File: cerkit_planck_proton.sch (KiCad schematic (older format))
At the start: 1 part

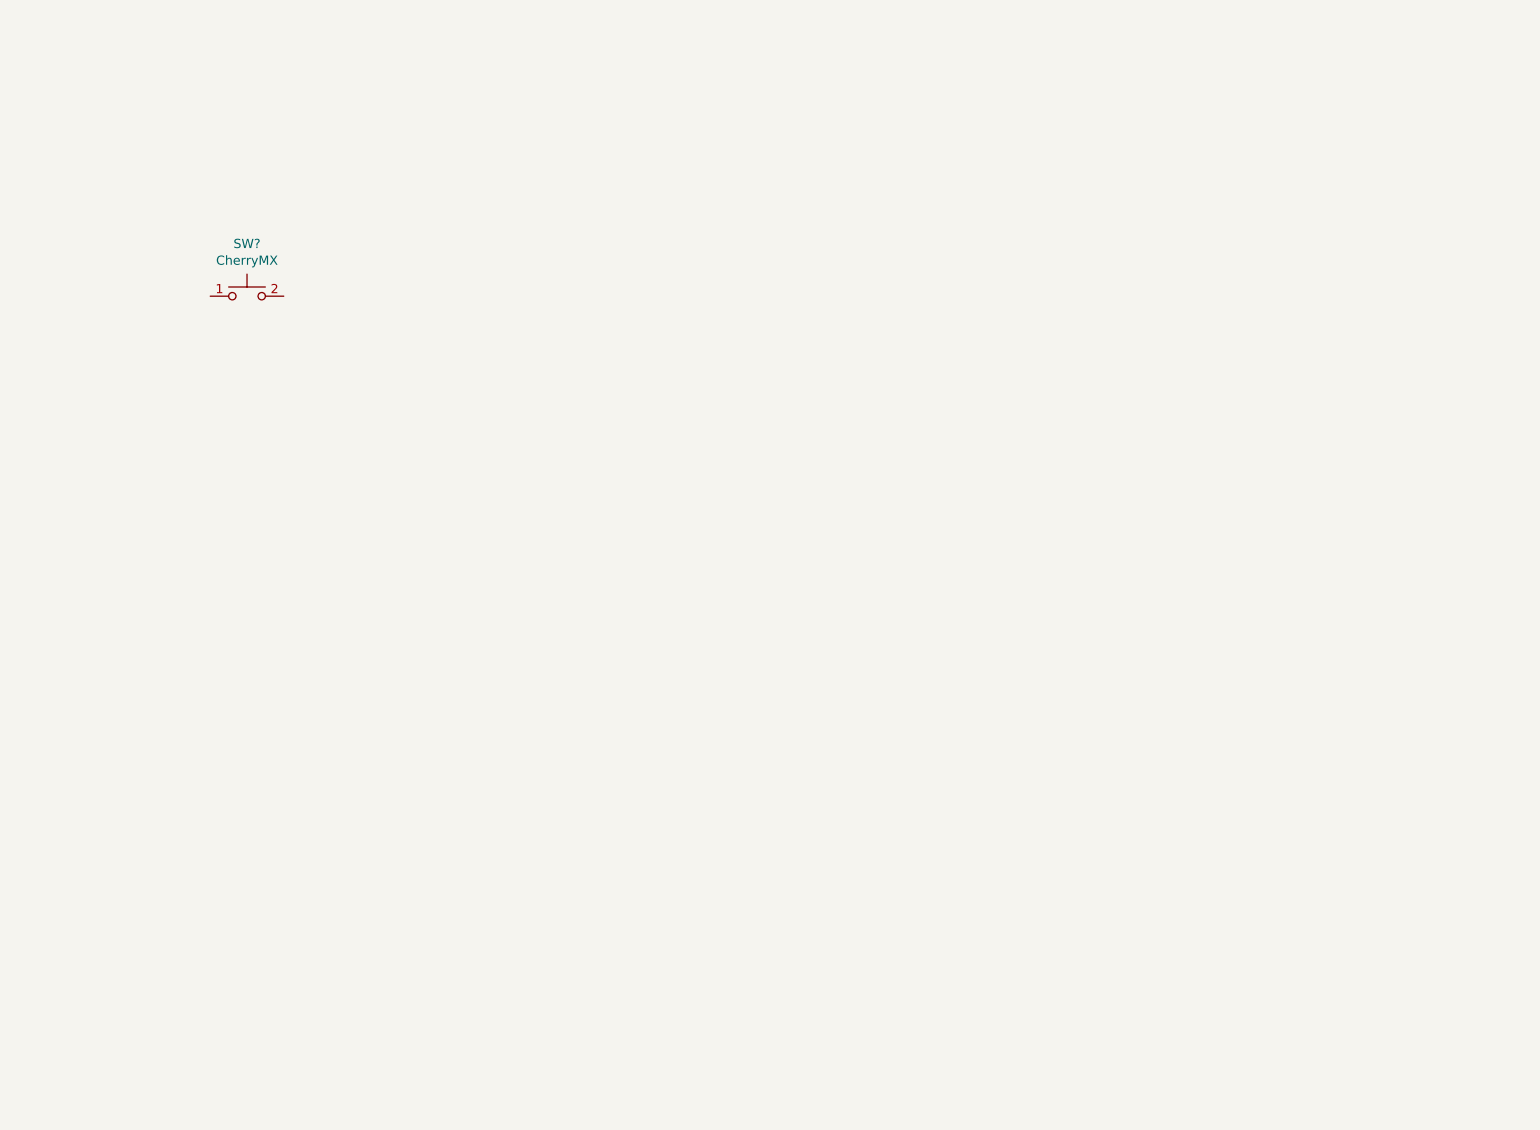
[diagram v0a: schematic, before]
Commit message: added schematic
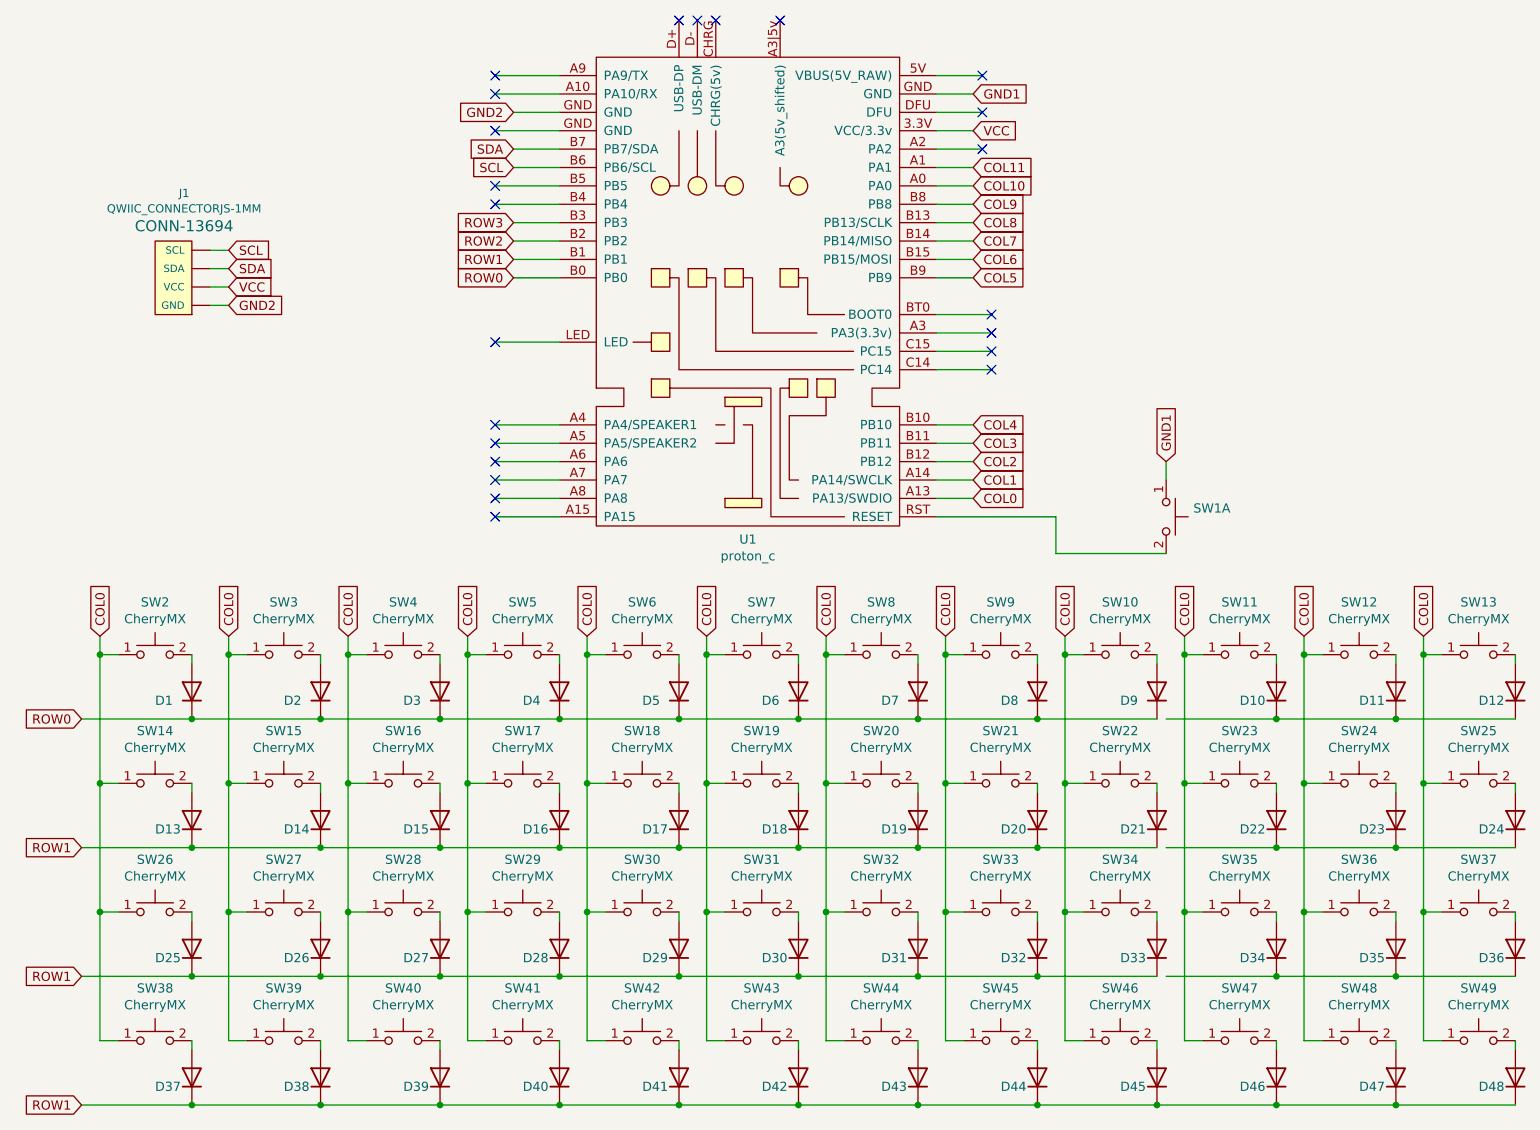
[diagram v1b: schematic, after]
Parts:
- added D1, D10, D11, D12, D13, D14, D15, D16, D17, D18, D19, D2, D20, D21, D22, D23, D24, D25, D26, D27, D28, D29, D3, D30, D31, D32, D33, D34, D35, D36, D37, D38, D39, D4, D40, D41, D42, D43, D44, D45, D46, D47, D48, D5, D6, D7, D8, D9: 1N4148, Diode_THT:D_DO-35_SOD27_P7.62mm_Horizontal, symbol Diode:1N4148
- added J1: QWIIC_CONNECTORJS-1MM, 1X04_1MM_RA, symbol SparkFun-Connectors:QWIIC_CONNECTORJS-1MM
- added SW1: SW_Push_Dual_x2, symbol Switch:SW_Push_Dual_x2
- added SW10, SW11, SW12, SW13, SW14, SW15, SW16, SW17, SW18, SW19, SW20, SW21, SW22, SW23, SW24, SW25, SW26, SW27, SW28, SW29, SW3, SW30, SW31, SW32, SW33, SW34, SW35, SW36, SW37, SW38, SW39, SW4, SW40, SW41, SW42, SW43, SW44, SW45, SW46, SW47, SW48, SW49, SW5, SW6, SW7, SW8, SW9: CherryMX, symbol CherryMX:CherryMX
- added U1: proton_c, symbol proton_c:proton_c
- gave numbers to parts that had none: 1
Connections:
- net COL0: now reaches SW2.1
- net COL0: now also SW10.1, SW11.1, SW12.1, SW13.1, SW14.1, SW15.1, SW16.1, SW17.1, SW18.1, SW19.1, SW20.1, SW21.1, SW22.1, SW23.1, SW24.1, SW25.1, SW26.1, SW27.1, SW28.1, SW29.1, SW3.1, SW30.1, SW31.1, SW32.1, SW33.1, SW34.1, SW35.1, SW36.1, SW37.1, SW38.1, SW39.1, SW4.1, SW40.1, SW41.1, SW42.1, SW43.1, SW44.1, SW45.1, SW46.1, SW47.1, SW48.1, SW49.1, SW5.1, SW6.1, SW7.1, SW8.1, SW9.1, U1.A13 (PA13/SWDIO)
- net at SW2.2: now also D1.2 (A)
- new net: D13.2 (A), SW14.2
- new net: D25.2 (A), SW26.2
- new net: D37.2 (A), SW38.2
- new net: SW1.2 (D), U1.RST (RESET)
- new net: D2.2 (A), SW3.2
- new net: D14.2 (A), SW15.2
- new net: D26.2 (A), SW27.2
- new net: D38.2 (A), SW39.2
- new net: D3.2 (A), SW4.2
- new net: D15.2 (A), SW16.2
- new net: D27.2 (A), SW28.2
- new net: D39.2 (A), SW40.2
- new net: D4.2 (A), SW5.2
- new net: D16.2 (A), SW17.2
- new net: D28.2 (A), SW29.2
- new net: D40.2 (A), SW41.2
- new net: D5.2 (A), SW6.2
- new net: D17.2 (A), SW18.2
- new net: D29.2 (A), SW30.2
- new net: D41.2 (A), SW42.2
- new net: D6.2 (A), SW7.2
- new net: D18.2 (A), SW19.2
- new net: D30.2 (A), SW31.2
- new net: D42.2 (A), SW43.2
- new net: D7.2 (A), SW8.2
- new net: D19.2 (A), SW20.2
- new net: D31.2 (A), SW32.2
- new net: D43.2 (A), SW44.2
- new net: D8.2 (A), SW9.2
- new net: D20.2 (A), SW21.2
- new net: D32.2 (A), SW33.2
- new net: D44.2 (A), SW45.2
- new net: D9.2 (A), SW10.2
- new net: D21.2 (A), SW22.2
- new net: D33.2 (A), SW34.2
- new net: D45.2 (A), SW46.2
- new net: D10.2 (A), SW11.2
- new net: D22.2 (A), SW23.2
- new net: D10.1 (K), D11.1 (K), D12.1 (K)
- new net: D22.1 (K), D23.1 (K), D24.1 (K)
- new net: D34.2 (A), SW35.2
- new net: D34.1 (K), D35.1 (K), D36.1 (K)
- new net: D46.2 (A), SW47.2
- new net: D11.2 (A), SW12.2
- new net: D23.2 (A), SW24.2
- new net: D35.2 (A), SW36.2
- new net: D47.2 (A), SW48.2
- new net: D12.2 (A), SW13.2
- new net: D24.2 (A), SW25.2
- new net: D36.2 (A), SW37.2
- new net: D48.2 (A), SW49.2
- new net COL1: U1.A14 (PA14/SWCLK)
- new net COL10: U1.A0 (PA0)
- new net COL11: U1.A1 (PA1)
- new net COL2: U1.B12 (PB12)
- new net COL3: U1.B11 (PB11)
- new net COL4: U1.B10 (PB10)
- new net COL5: U1.B9 (PB9)
- new net COL6: U1.B15 (PB15/MOSI)
- new net COL7: U1.B14 (PB14/MISO)
- new net COL8: U1.B13 (PB13/SCLK)
- new net COL9: U1.B8 (PB8)
- new net GND1: SW1.1 (C), U1.GND
- new net GND2: J1.1 (GND), U1.GND
- new net ROW0: D1.1 (K), D2.1 (K), D3.1 (K), D4.1 (K), D5.1 (K), D6.1 (K), D7.1 (K), D8.1 (K), D9.1 (K), U1.B0 (PB0)
- new net ROW1: D13.1 (K), D14.1 (K), D15.1 (K), D16.1 (K), D17.1 (K), D18.1 (K), D19.1 (K), D20.1 (K), D21.1 (K), D25.1 (K), D26.1 (K), D27.1 (K), D28.1 (K), D29.1 (K), D30.1 (K), D31.1 (K), D32.1 (K), D33.1 (K), D37.1 (K), D38.1 (K), D39.1 (K), D40.1 (K), D41.1 (K), D42.1 (K), D43.1 (K), D44.1 (K), D45.1 (K), D46.1 (K), D47.1 (K), D48.1 (K), U1.B1 (PB1)
- new net ROW2: U1.B2 (PB2)
- new net ROW3: U1.B3 (PB3)
- new net SCL: J1.4 (SCL), U1.B6 (PB6/SCL)
- new net SDA: J1.3 (SDA), U1.B7 (PB7/SDA)
- new net VCC: J1.2 (VCC), U1.3.3V (VCC/3.3v)
- no-connect marks 0 -> 23
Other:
- moved on the sheet: SW2
